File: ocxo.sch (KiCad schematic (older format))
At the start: 21 parts, among them J1 Conn_01x02, J2 Conn_01x01, J3 Conn_Coaxial, J4 Conn_01x01, J5 Conn_01x01, J6 Conn_01x01, J7 Conn_Coaxial, Q1 ENE3311 OCXO, U1 KA78M05_TO252, U2 LM4140

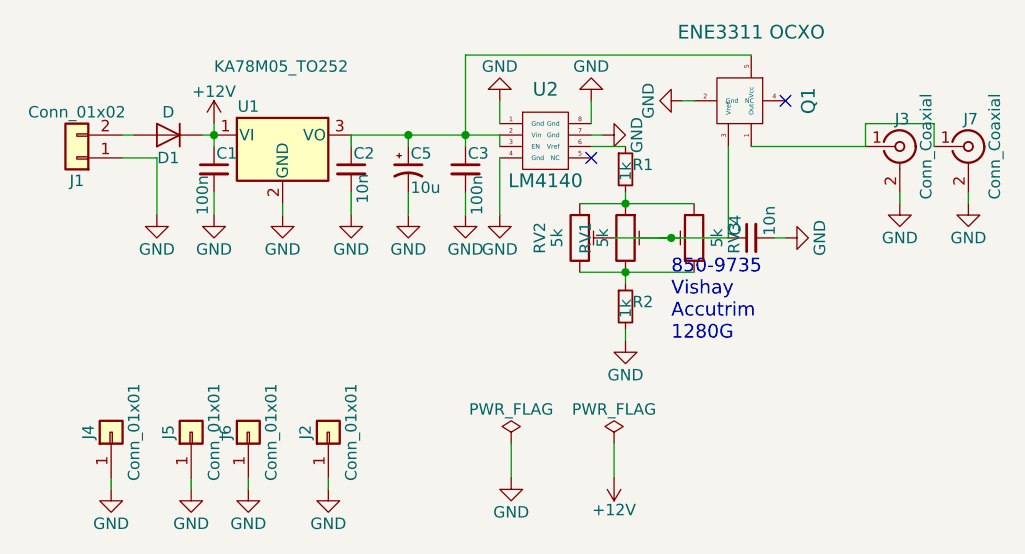
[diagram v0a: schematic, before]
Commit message: minor bug fixed
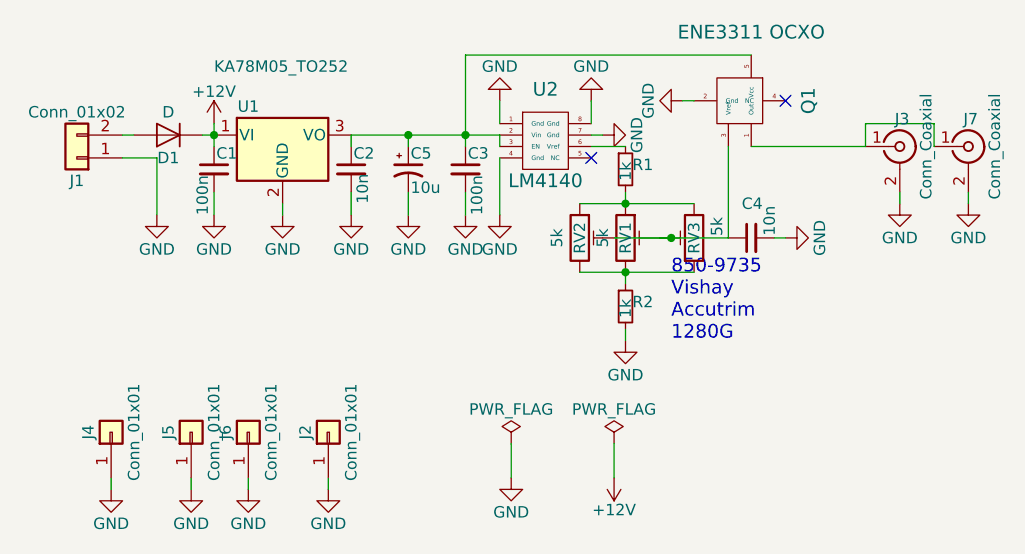
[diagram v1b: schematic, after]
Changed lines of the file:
@@
 U 1 1 5A0B6442
 P 4250 2000
-F 0 "RV1" V 4075 2000 50  0000 C CNN
+F 0 "RV1" V 4250 2000 50  0000 C CNN
 F 1 "5k" V 4150 2000 50  0000 C CNN
 F 2 "Potentiometers:Potentiometer_Trimmer_Vishay_43" H 4250 2000 50  0001 C CNN
@@
 U 1 1 5A0B664E
 P 4800 2000
-F 0 "C4" H 4810 2070 50  0000 L CNN
+F 0 "C4" V 4950 1950 50  0000 L CNN
 F 1 "10n" H 4810 1920 50  0000 L CNN
 F 2 "Capacitors_SMD:C_0805_HandSoldering" H 4800 2000 50  0001 C CNN
@@
 U 1 1 5A425F65
 P 4050 2000
-F 0 "RV2" V 3875 2000 50  0000 C CNN
+F 0 "RV2" V 4050 2000 50  0000 C CNN
 F 1 "5k" V 3950 2000 50  0000 C CNN
 F 2 "Potentiometers:Potentiometer_Trimmer_Bourns_3299Y" H 4050 2000 50  0001 C CNN
@@
 U 1 1 5A426460
 P 4550 2000
-F 0 "RV3" V 4375 2000 50  0000 C CNN
-F 1 "5k" V 4450 2000 50  0000 C CNN
+F 0 "RV3" V 4550 2000 50  0000 C CNN
+F 1 "5k" V 4450 1950 50  0000 C CNN
 F 2 "Potentiometers:Potentiometer_Trimmer_Bourns_3299W" H 4550 2000 50  0001 C CNN
 F 3 "" H 4550 2000 50  0001 C CNN
